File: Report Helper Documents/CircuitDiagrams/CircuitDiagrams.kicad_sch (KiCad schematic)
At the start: 6 parts

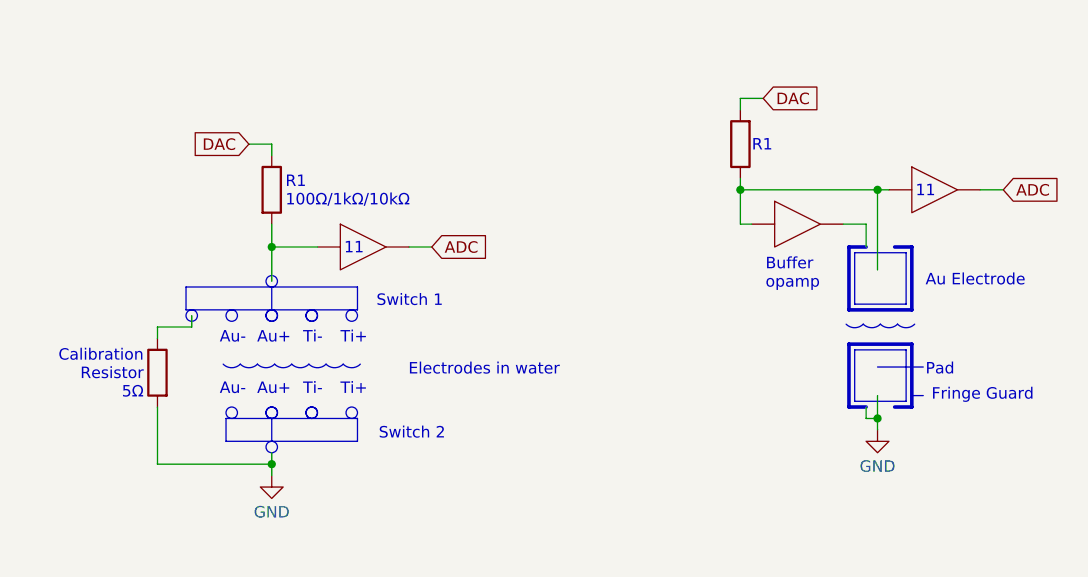
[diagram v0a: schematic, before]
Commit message: report writing
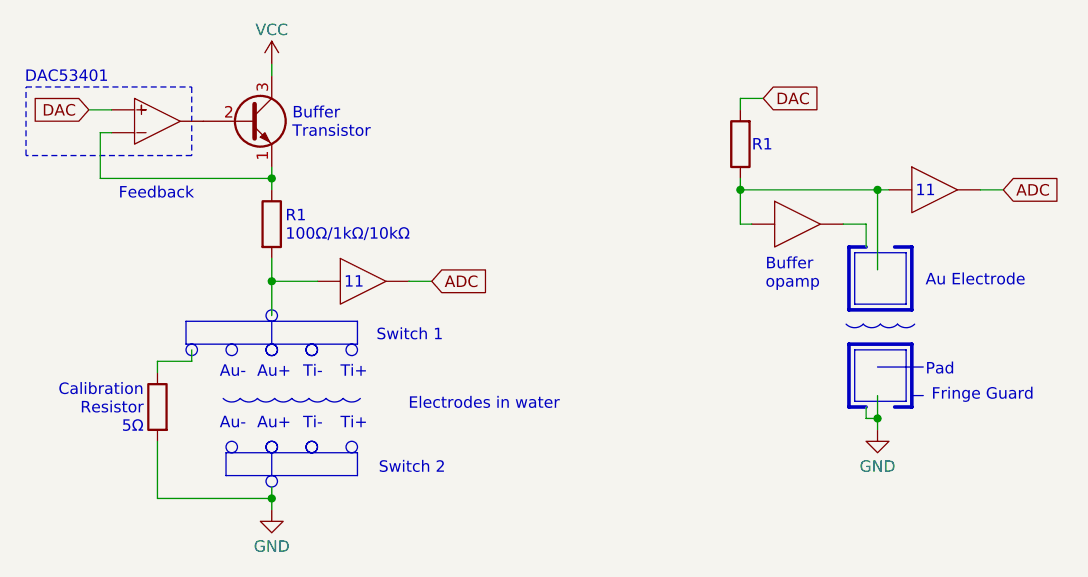
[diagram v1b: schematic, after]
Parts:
- added Q1: 2N2219, Package_TO_SOT_THT:TO-39-3, symbol Transistor_BJT:2N2219
- added U4: ~, symbol 4022S:OPAMP_PM
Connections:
- net DAC: now also U4.; no longer R1.1
- new net: Q1.1 (E), R1.1, U4.
- new net: Q1.2 (B), U4.
- new net: R2.1, U2., U3.
- new net VCC: Q1.3 (C)
- now unconnected: U2.
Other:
- note added: "Buffer Transistor"
- note added: "DAC53401"
- note added: "Feedback"
